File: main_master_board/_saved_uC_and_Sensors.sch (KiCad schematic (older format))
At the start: 2 parts, among them U15 DSPIC33EP512GP806-I/PT

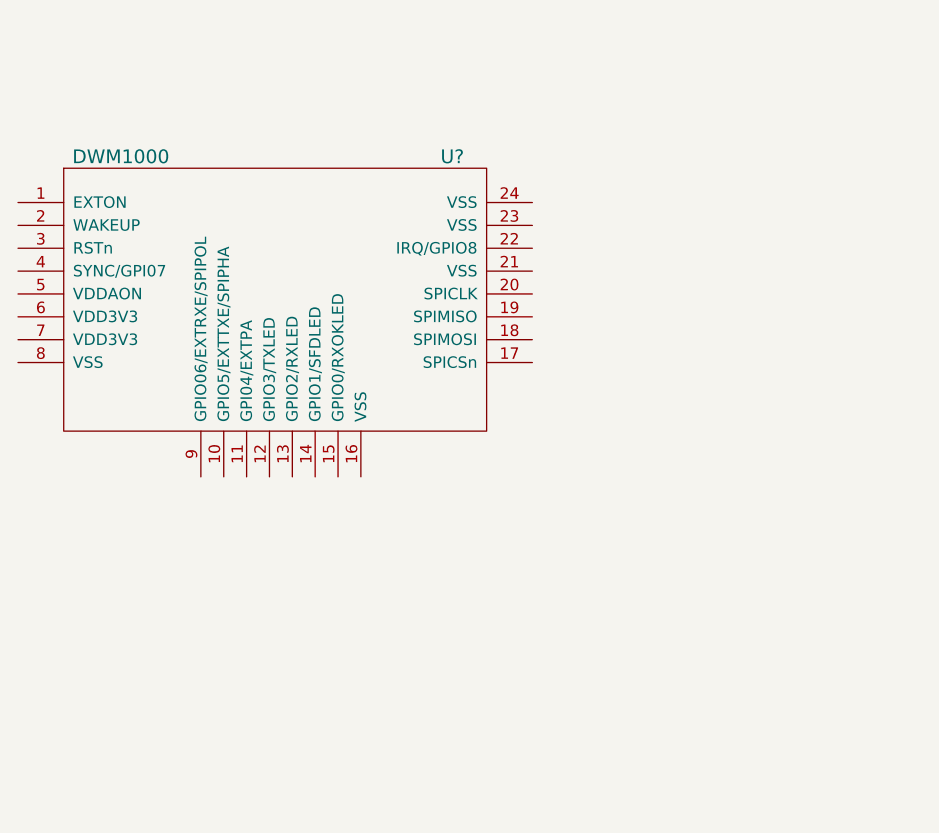
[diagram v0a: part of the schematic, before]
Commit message: I did a lot of things
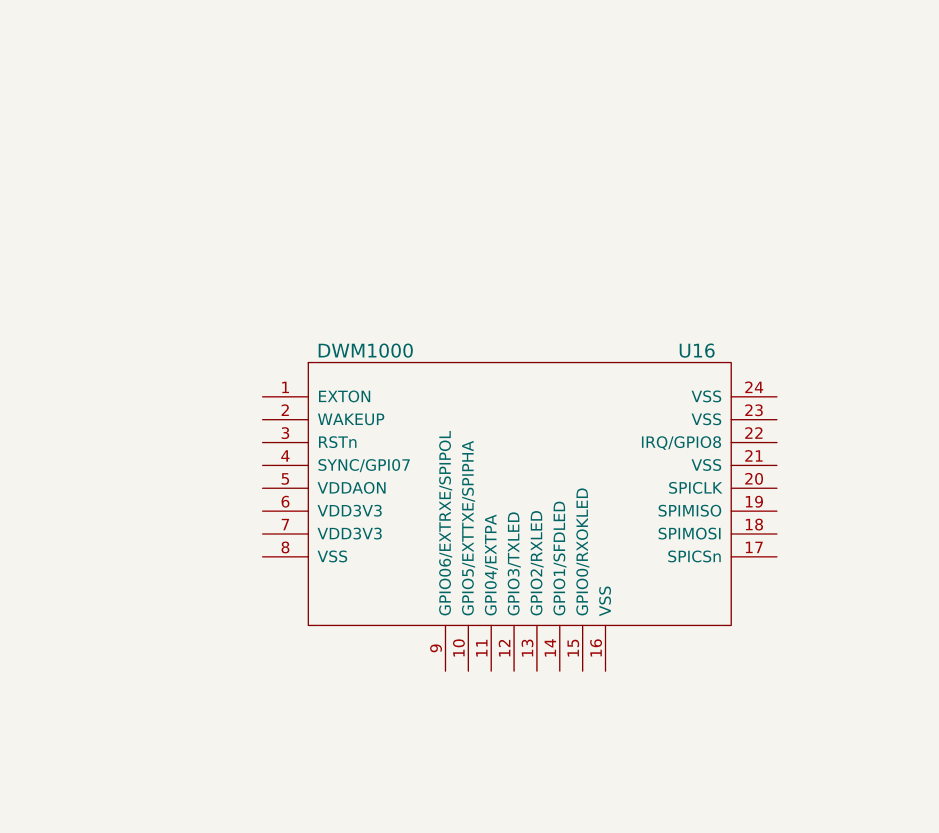
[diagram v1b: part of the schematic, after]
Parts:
- U16: renamed from U?; footprint (none) -> decaWave:dmw1000
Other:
- moved on the sheet: U16
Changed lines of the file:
@@
 $EndComp
 $Comp
-L DWM1000 U?
+L DWM1000 U16
 U 1 1 58782FE7
-P 3400 3740
-F 0 "U?" H 4150 4840 60  0000 C CNN
-F 1 "DWM1000" H 2700 4840 60  0000 C CNN
-F 2 "" H 3400 3790 60  0000 C CNN
-F 3 "" H 3400 3790 60  0000 C CNN
-	1    3400 3740
+P 4470 4590
+F 0 "U16" H 5220 5690 60  0000 C CNN
+F 1 "DWM1000" H 3770 5690 60  0000 C CNN
+F 2 "decaWave:dmw1000" H 4470 4640 60  0001 C CNN
+F 3 "" H 4470 4640 60  0000 C CNN
+	1    4470 4590
 	1    0    0    -1
 $EndComp
